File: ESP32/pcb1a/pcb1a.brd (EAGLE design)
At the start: 68.9 x 63.5 mm, 13 parts

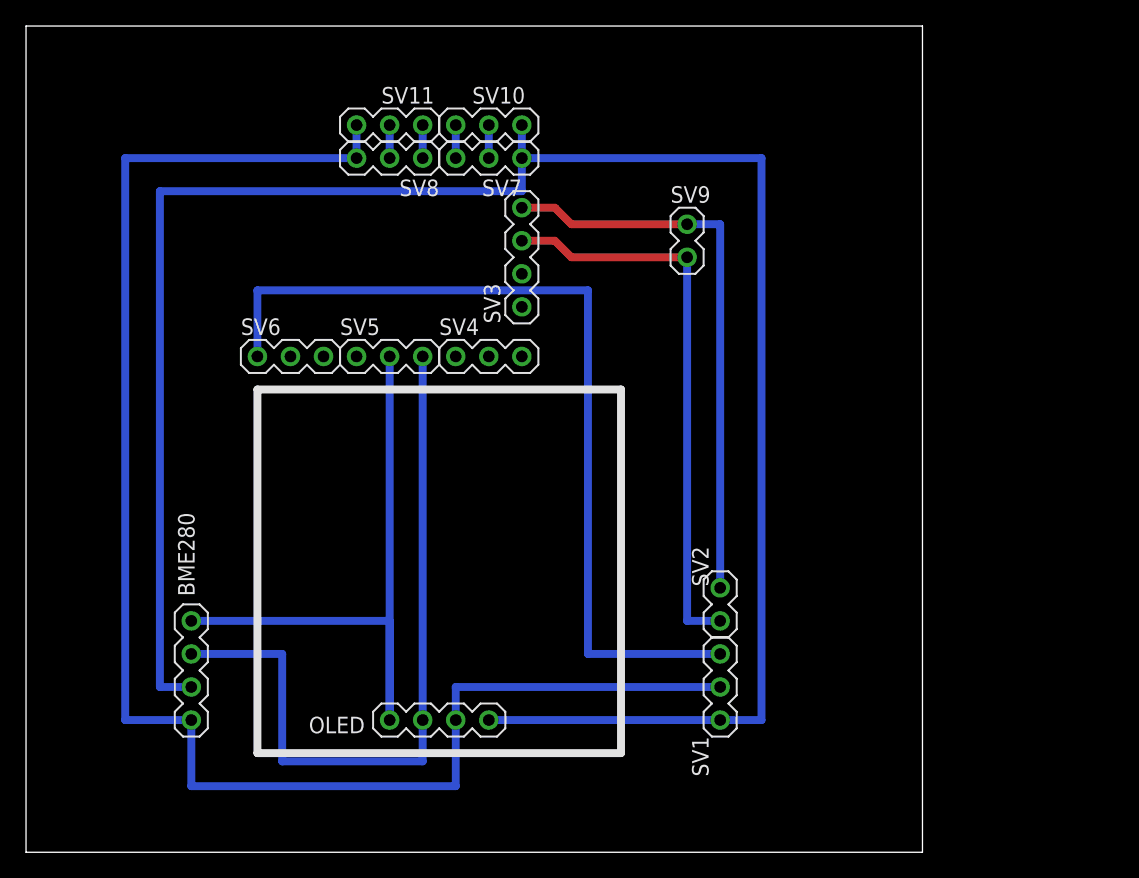
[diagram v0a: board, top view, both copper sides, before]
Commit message: UPD: ESP32/pcb1a/
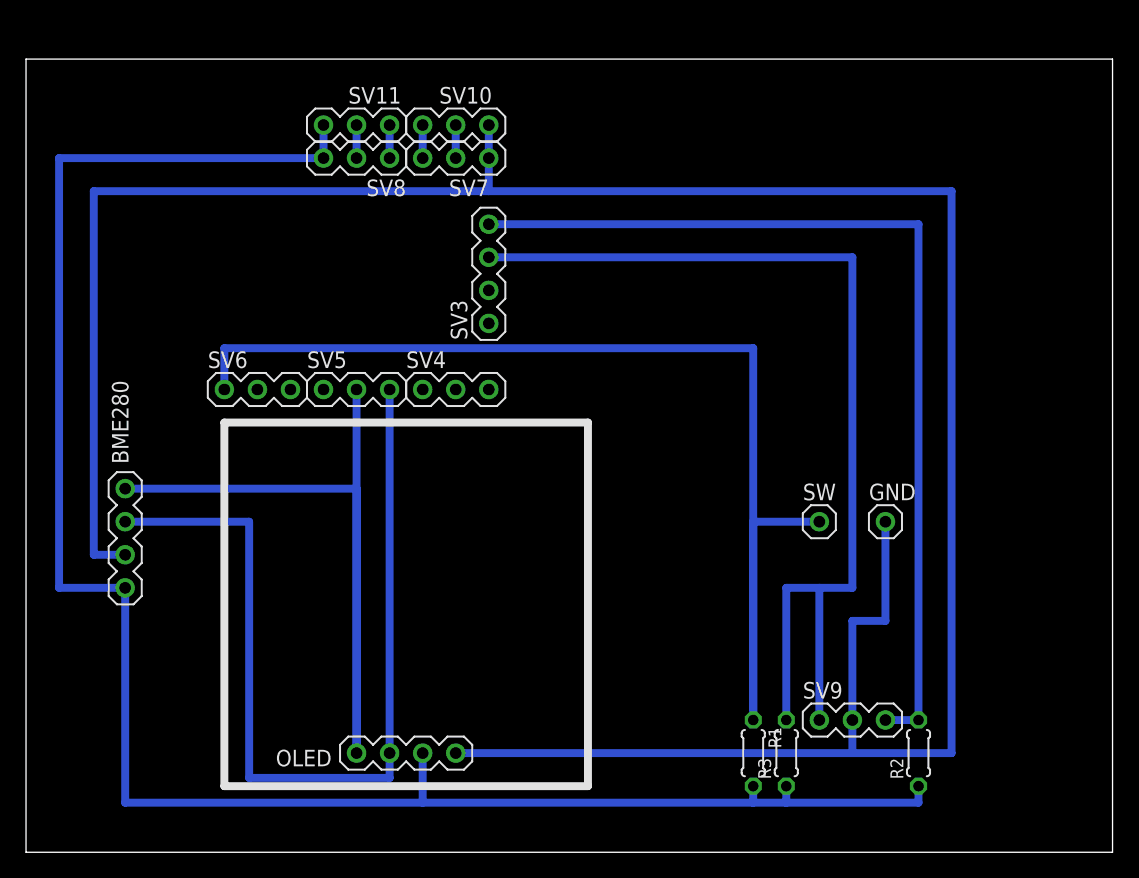
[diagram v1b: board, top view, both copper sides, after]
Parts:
- removed SV1: (no value), ytani1:PINHEAD-MA03-1
- removed SV2: (no value), ytani1:PINHEAD-MA02-1
- added GND, SW: (no value), ytani1:PINHEAD-MA01-1
- added R1, R2, R3: 10K, rcl:0204/5
- SV9: device ytani1:PINHEAD-MA02-1 -> ytani1:PINHEAD-MA03-1
- moved SV9 38.6 mm to (62.2, 10.2), turned to 0 degrees
- moved BME280 11.4 mm to (7.62, 24.1)
- moved SV5 3.59 mm to (24.1, 35.6)
- moved OLED 3.59 mm to (29.2, 7.62)
- moved SV4 3.59 mm to (31.8, 35.6)
- moved SV6 3.59 mm to (16.5, 35.6)
- moved SV3 2.84 mm to (35.6, 44.5)
- moved SV10 2.54 mm to (34.3, 55.9)
- moved SV11 2.54 mm to (26.7, 55.9)
- moved SV7 2.54 mm to (34.3, 53.3)
- moved SV8 2.54 mm to (26.7, 53.3)
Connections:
- removed net N$5: SV2.2, SV3.4, SV9.2
- new net N$10: R1.1, SV6.1, SW.1
- net +3V3: now also R1.2, R2.1, R3.1; no longer SV1.2
- net GND: now also GND.1, SV9.2; no longer SV1.1
- net N$1: now also R3.2, SV3.3, SV9.1; no longer SV1.3, SV6.1
- net N$6: now also R2.2, SV3.4, SV9.3; no longer SV2.1, SV3.3, SV9.1
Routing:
- net N$10: track 0.00 -> 92.7 mm
- net GND: track 156.0 -> 202.9 mm
- net N$5: track 43.7 -> 0.00 mm
- net N$6: track 43.7 -> 73.7 mm
- net +3V3: track 121.9 -> 146.1 mm
- net N$3: track 50.8 -> 66.0 mm
- net N$2: track 57.1 -> 69.8 mm
- net N$1: track 68.6 -> 78.7 mm
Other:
- board size 68.9 x 63.5 mm -> 83.5 x 61 mm
